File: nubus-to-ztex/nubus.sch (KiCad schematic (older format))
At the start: 56 parts, among them J4 C96ABC, U1 74LVT125, U2 74LVT125, U3 74LVT125, U4 XC9572XL-VQ64, U5 74LVT245BPW,118, U6 74LVT245BPW,118, U7 74LVT245BPW,118, U8 74LVT245BPW,118

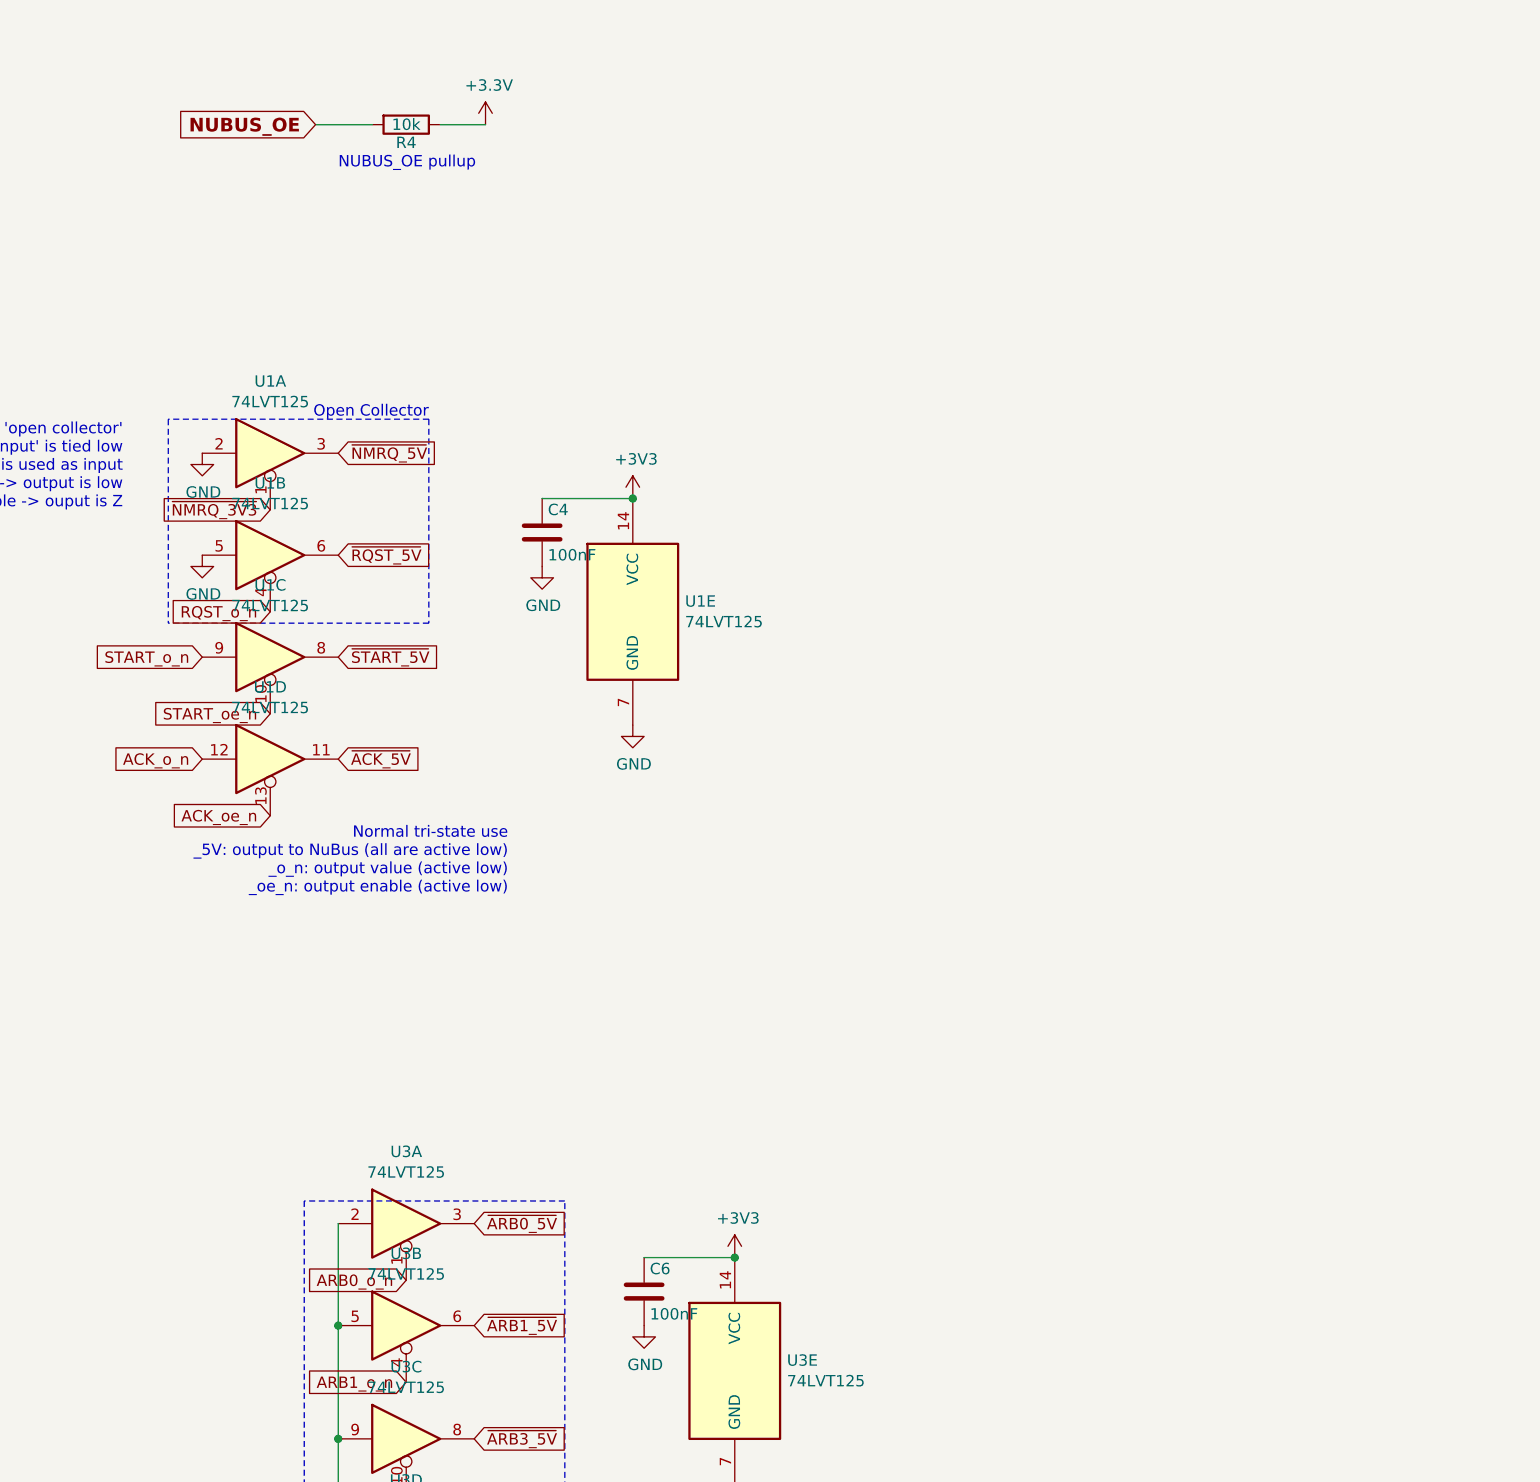
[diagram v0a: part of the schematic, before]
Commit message: more updates
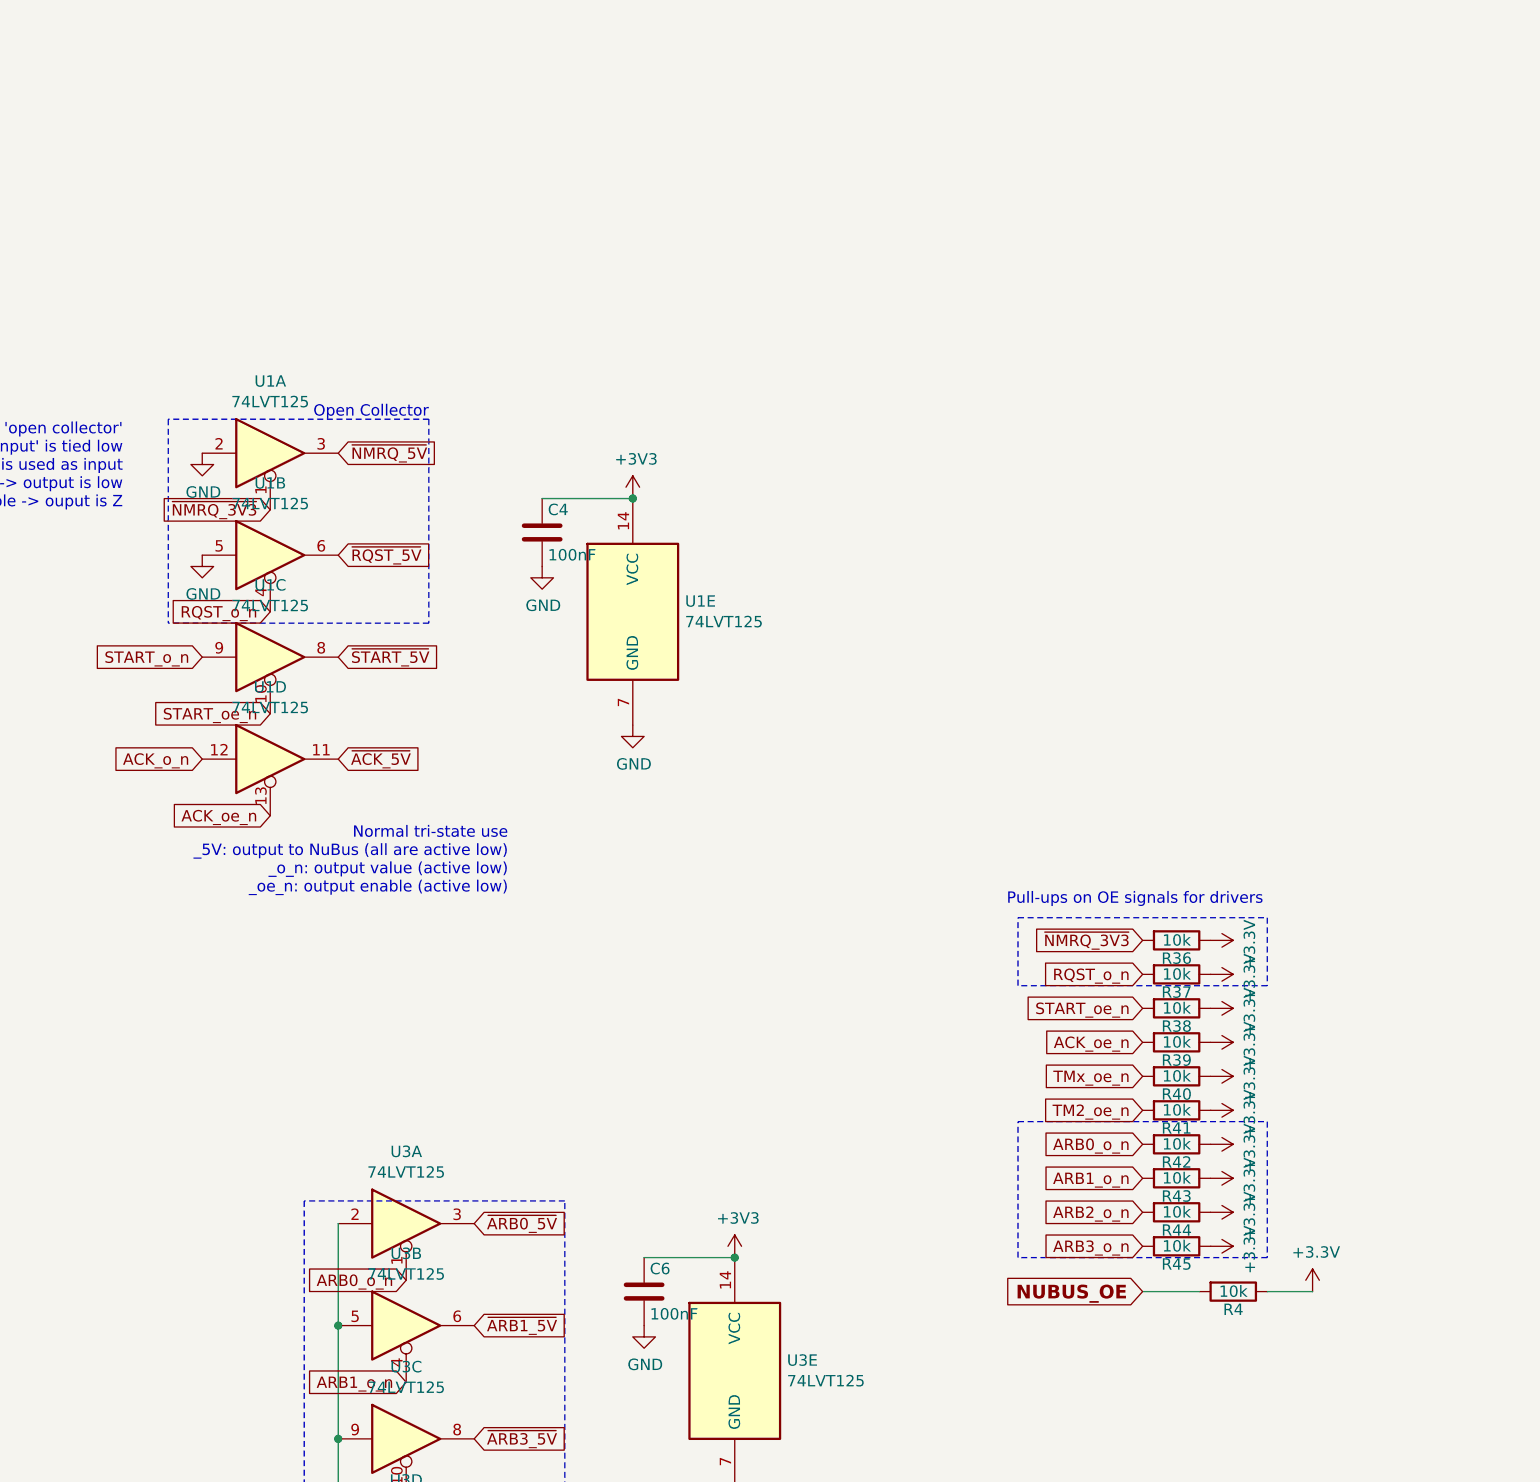
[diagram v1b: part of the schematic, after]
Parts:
- added R36, R37, R38, R39, R40, R41, R42, R43, R44, R45: 10k, Resistor_SMD:R_0603_1608Metric, symbol Device:R
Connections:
- net +3V3: now also R36.1, R37.1, R38.1, R39.1, R40.1, R41.1, R42.1, R43.1, R44.1, R45.1
- net ACK_oe_n: now also R39.2
- net ARB0_o_n: now also R42.2
- net ARB1_o_n: now also R43.2
- net ARB2_o_n: now also R44.2
- net ARB3_o_n: now also R45.2
- net RQST_o_n: now also R37.2
- net START_oe_n: now also R38.2
- net TM2_oe_n: now also R41.2
- net TMx_oe_n: now also R40.2
- net ~NMRQ_3V3: now also R36.2
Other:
- note added: "Pull-ups on OE signals for drivers"
- note removed: "NUBUS_OE pullup"
- moved on the sheet: R4

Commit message: some missing stuff, minor HW update, SW
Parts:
- U5, U6, U7, U8: URL https://eu.mouser.com/ProductDetail/?qs=me8TqzrmIYVnC5%252B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 -> https://www.digikey.fr/fr/products/detail/nexperia-usa-inc/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; URL-mouser (none) -> https://eu.mouser.com/ProductDetail/?qs=me8TqzrmIYVnC5%252B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
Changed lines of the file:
@@
 F 2 "For_SeeedStudio:TSSOP-20_4.4x6.5mm_P0.65mm_ForSeeedStudio" H 17350 3450 50  0001 C CNN
 F 3 "http://www.ti.com/lit/gpn/sn74LS245" H 17350 3450 50  0001 C CNN
-F 4 "https://eu.mouser.com/ProductDetail/?qs=me8TqzrmIYVnC5%252BK4SaiTg%3D%3D" H 17350 3450 50  0001 C CNN "URL"
+F 4 "https://eu.mouser.com/ProductDetail/?qs=me8TqzrmIYVnC5%252BK4SaiTg%3D%3D" H 17350 3450 50  0001 C CNN "URL-mouser"
 F 5 "74LVT245BPW,118" H 17350 3450 50  0001 C CNN "MPN"
+F 6 "https://www.digikey.fr/fr/products/detail/nexperia-usa-inc/74LVT245BPW-118/1231957" H 17350 3450 50  0001 C CNN "URL"
 	1    17350 3450
 	-1   0    0    -1
@@
 F 3 "http://www.ti.com/lit/gpn/sn74LS245" H 15350 3450 50  0001 C CNN
 F 4 "74LVT245BPW,118" H 15350 3450 50  0001 C CNN "MPN"
-F 5 "https://eu.mouser.com/ProductDetail/?qs=me8TqzrmIYVnC5%252BK4SaiTg%3D%3D" H 15350 3450 50  0001 C CNN "URL"
+F 5 "https://eu.mouser.com/ProductDetail/?qs=me8TqzrmIYVnC5%252BK4SaiTg%3D%3D" H 15350 3450 50  0001 C CNN "URL-mouser"
+F 6 "https://www.digikey.fr/fr/products/detail/nexperia-usa-inc/74LVT245BPW-118/1231957" H 15350 3450 50  0001 C CNN "URL"
 	1    15350 3450
 	-1   0    0    -1
@@
 F 3 "http://www.ti.com/lit/gpn/sn74LS245" H 13300 3450 50  0001 C CNN
 F 4 "74LVT245BPW,118" H 13300 3450 50  0001 C CNN "MPN"
-F 5 "https://eu.mouser.com/ProductDetail/?qs=me8TqzrmIYVnC5%252BK4SaiTg%3D%3D" H 13300 3450 50  0001 C CNN "URL"
+F 5 "https://eu.mouser.com/ProductDetail/?qs=me8TqzrmIYVnC5%252BK4SaiTg%3D%3D" H 13300 3450 50  0001 C CNN "URL-mouser"
+F 6 "https://www.digikey.fr/fr/products/detail/nexperia-usa-inc/74LVT245BPW-118/1231957" H 13300 3450 50  0001 C CNN "URL"
 	1    13300 3450
 	-1   0    0    -1
@@
 F 3 "http://www.ti.com/lit/gpn/sn74LS245" H 11250 3450 50  0001 C CNN
 F 4 "74LVT245BPW,118" H 11250 3450 50  0001 C CNN "MPN"
-F 5 "https://eu.mouser.com/ProductDetail/?qs=me8TqzrmIYVnC5%252BK4SaiTg%3D%3D" H 11250 3450 50  0001 C CNN "URL"
+F 5 "https://eu.mouser.com/ProductDetail/?qs=me8TqzrmIYVnC5%252BK4SaiTg%3D%3D" H 11250 3450 50  0001 C CNN "URL-mouser"
 F 6 "https://www.renesas.com/us/en/package/pcg20" H 11250 3450 50  0001 C CNN "Drawings"
 F 7 "https://www.renesas.com/document/psc/pcpcg-package-outline-150-body-width-qsop-025-pitch?language=en" H 11250 3450 50  0001 C CNN "Datasheet - Packaging"
 F 8 "https://assets.nexperia.com/documents/package-information/SOT360-1.pdf" H 11250 3450 50  0001 C CNN "Package Drawings"
+F 9 "https://www.digikey.fr/fr/products/detail/nexperia-usa-inc/74LVT245BPW-118/1231957" H 11250 3450 50  0001 C CNN "URL"
 	1    11250 3450
 	-1   0    0    -1
